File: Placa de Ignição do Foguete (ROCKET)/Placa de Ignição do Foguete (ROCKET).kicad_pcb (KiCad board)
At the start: 2 copper layers, 9 parts, among them J1 Bateria ESP, J3 Squibes, Q1 Q_NMOS_GDS, U1 ESP32-DEVKITC-32E, U2 RA-02_LORA

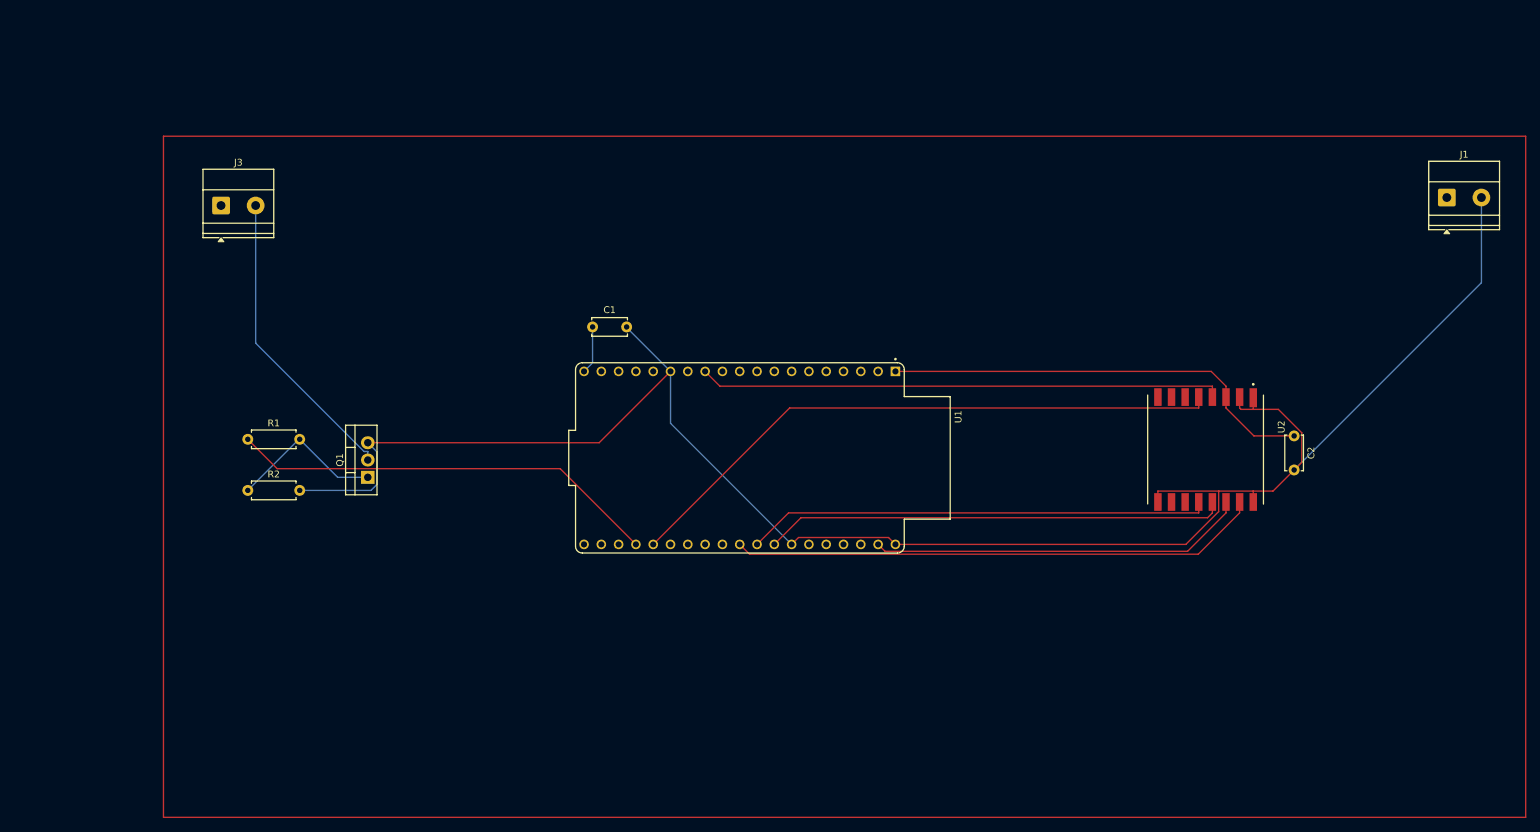
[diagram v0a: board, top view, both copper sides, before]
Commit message: to loco
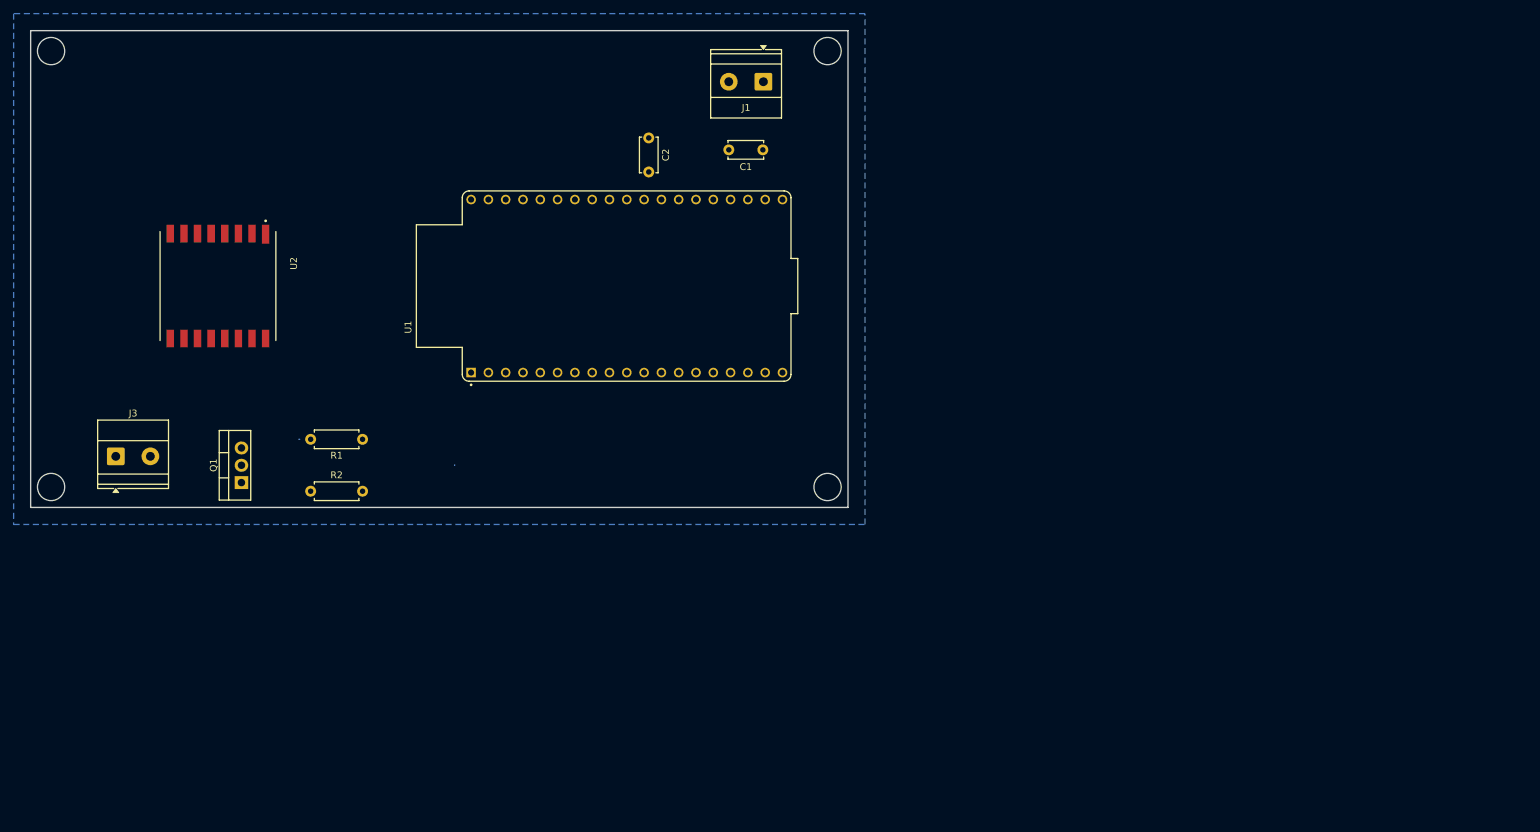
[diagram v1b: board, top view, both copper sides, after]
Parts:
- moved U2 147.0 mm to (47.5, 57.5)
- moved C2 104.4 mm to (110.8, 35.8)
- moved J1 101.8 mm to (127.6, 27.5), turned to 180 degrees
- moved J3 39.9 mm to (32.5, 82.5)
- moved C1 36.1 mm to (127.5, 37.5), turned to 180 degrees
- moved U1 30.2 mm to (107.5, 57.5), turned to 90 degrees
- moved Q1 18.6 mm to (51.0, 86.3)
- moved R1 16.9 mm to (68.7, 80.0), turned to 180 degrees
- moved R2 9.23 mm to (61.1, 87.6)
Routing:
- net GND: track 273.4 -> 0.08 mm
- net /DIO0 (LoRa): track 90.0 -> 0.00 mm
- net /NSS / CS (LoRa): track 78.1 -> 0.00 mm
- net /RST (LoRa): track 77.0 -> 0.00 mm
- net /SCK (LoRa): track 68.4 -> 0.00 mm
- net /MISO (LoRa): track 67.8 -> 0.00 mm
- net /3V3: track 64.3 -> 0.00 mm
- net /GATE_CTRL: track 63.4 -> 0.00 mm
- net /MOSI (LoRa): track 55.4 -> 0.00 mm
- net /SQUIBES_OUT: track 44.5 -> 0.00 mm
- net Net-(Q1-G): track 23.0 -> 0.12 mm
- net /VCC: track 7.05 -> 0.00 mm
- added copper zone on B.Cu, net GND
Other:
- board outline added: 120 x 70 mm
